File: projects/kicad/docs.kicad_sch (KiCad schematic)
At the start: 19 parts, among them SW1 SW_PUSH, SW2 SW_PUSH, SW3 SW_PUSH, SW4 SW_PUSH, SW5 SW_PUSH, SW6 SW_PUSH, SW7 RotaryEncoder_Switch, U1 Pico, U3 2.8_240x320_touch_sd_spi

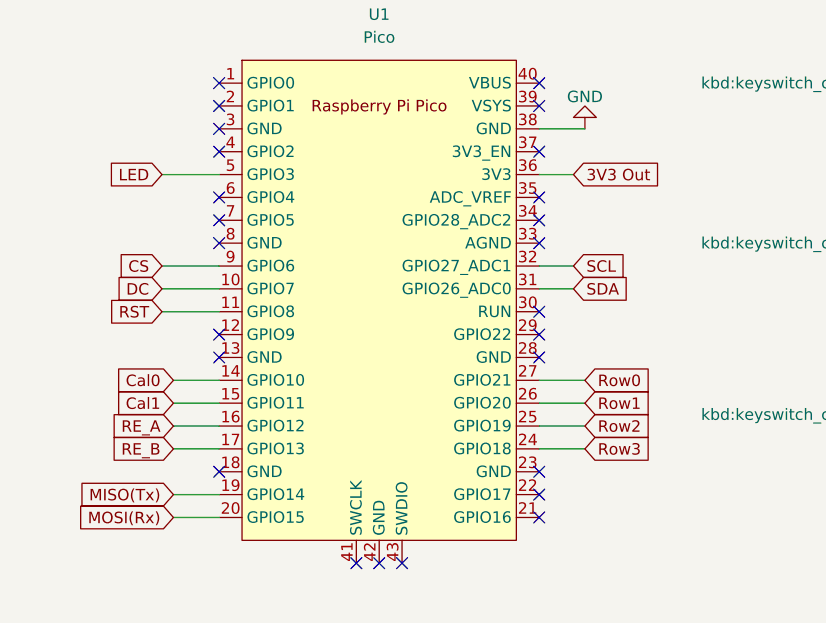
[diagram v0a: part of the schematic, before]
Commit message: Update_0129_yamaguchi
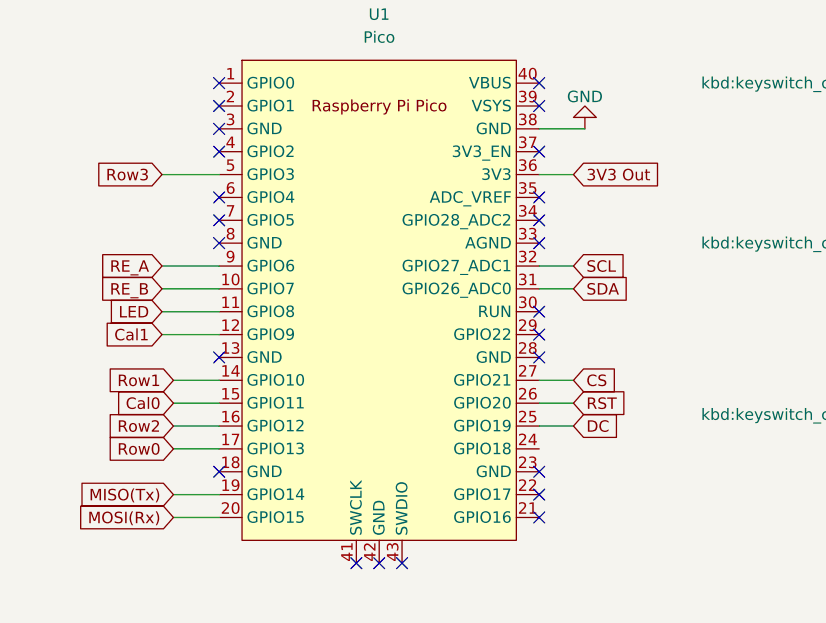
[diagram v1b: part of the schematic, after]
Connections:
- net CS: now also U1.27 (GPIO21); no longer U1.9 (GPIO6)
- net Cal0: now also U1.15 (GPIO11); no longer U1.14 (GPIO10)
- net Cal1: now also U1.12 (GPIO9); no longer U1.15 (GPIO11)
- net DC: now also U1.25 (GPIO19); no longer U1.10 (GPIO7)
- net LED: now also U1.11 (GPIO8); no longer U1.5 (GPIO3)
- net RE_A: now also U1.9 (GPIO6); no longer U1.16 (GPIO12)
- net RE_B: now also U1.10 (GPIO7); no longer U1.17 (GPIO13)
- net RST: now also U1.26 (GPIO20); no longer U1.11 (GPIO8)
- net Row0: now also U1.17 (GPIO13); no longer U1.27 (GPIO21)
- net Row1: now also U1.14 (GPIO10); no longer U1.26 (GPIO20)
- net Row2: now also U1.16 (GPIO12); no longer U1.25 (GPIO19)
- net Row3: now also U1.5 (GPIO3); no longer U1.24 (GPIO18)
- no-connect marks 28 -> 27
